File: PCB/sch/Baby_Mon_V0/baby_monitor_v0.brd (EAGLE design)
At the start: 22.8 x 16.2 mm, 2 parts, among them U1 NRF5340-QKAA-AB0-R

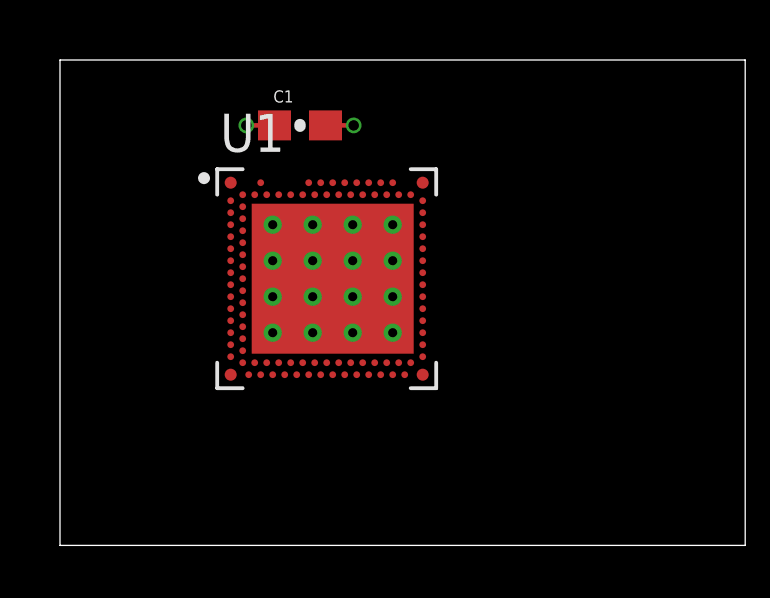
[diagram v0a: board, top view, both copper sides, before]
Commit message: u
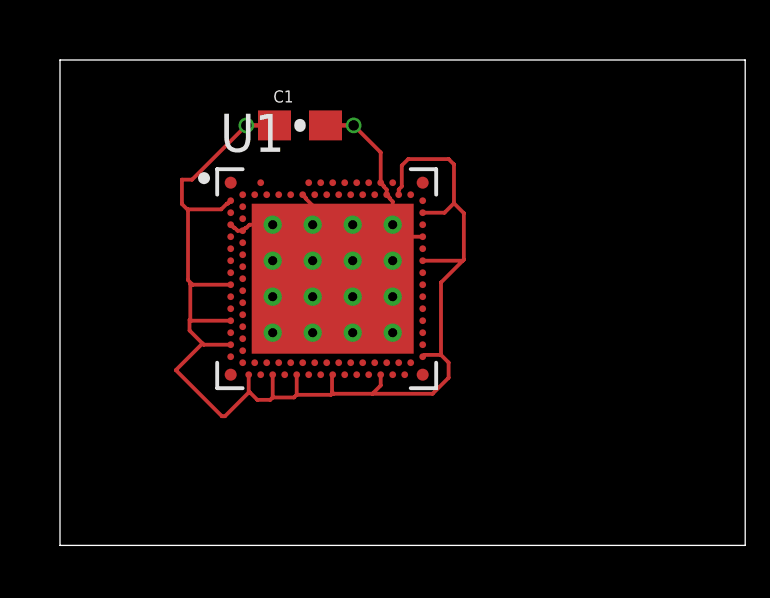
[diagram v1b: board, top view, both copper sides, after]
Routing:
- net 3.3V: track 0.94 -> 43.9 mm
- net GND: track 0.94 -> 8.66 mm

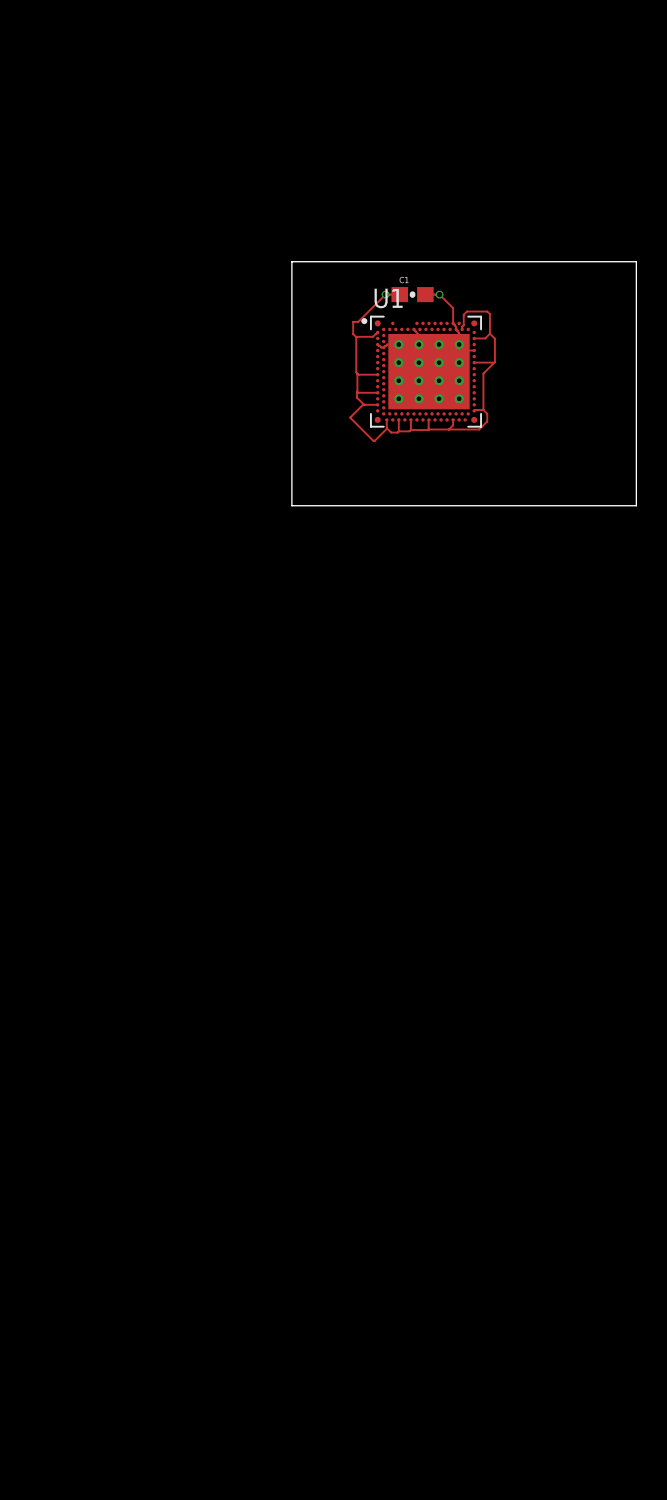
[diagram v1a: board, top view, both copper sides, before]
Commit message: u
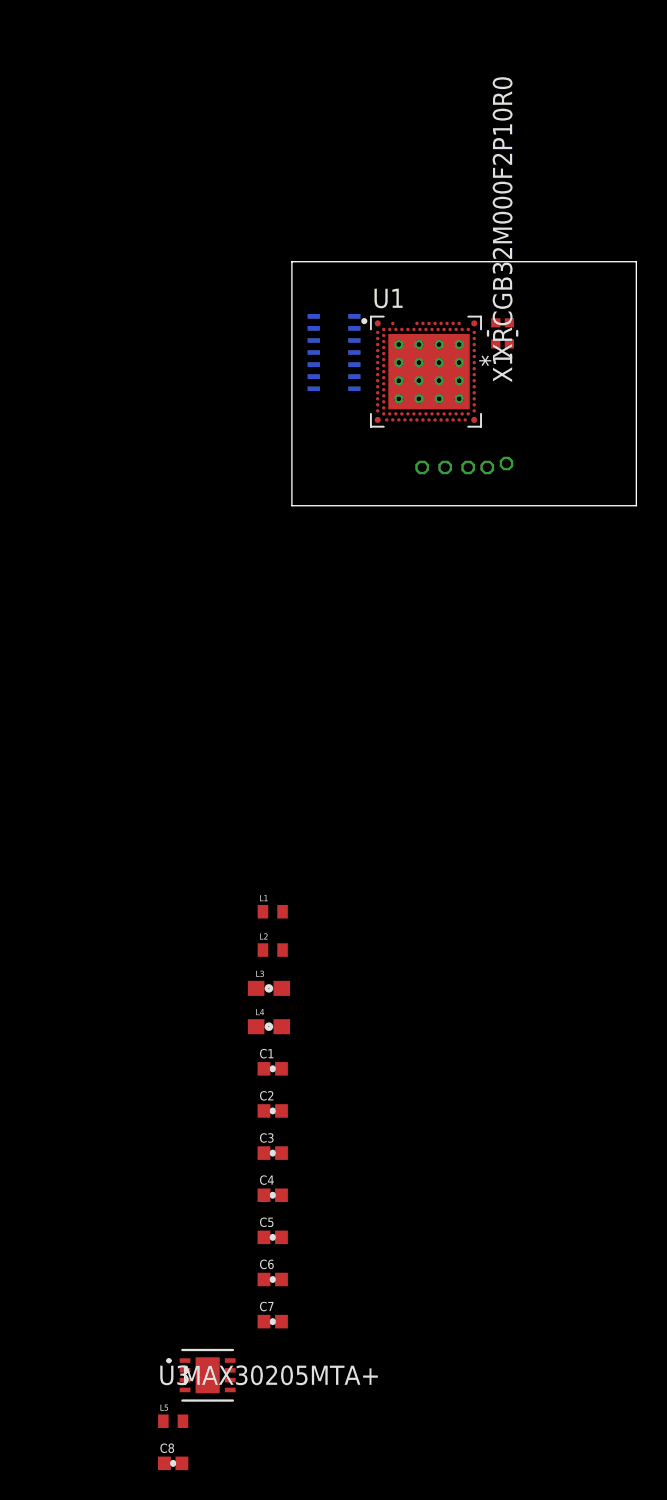
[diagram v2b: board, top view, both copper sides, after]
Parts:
- added C2, C6: 1uF, SparkFun-Capacitors:0402-CAP
- added C3: 1.0uF, SparkFun-Capacitors:0402-CAP
- added C4, C5, C7: 0.1uF, SparkFun-Capacitors:0402-CAP
- added C8: 0.7pF, SparkFun-Capacitors:0402-CAP
- added FRAME1, FRAME2, FRAME3: FRAME-LETTERNO_PACKAGE, SparkFun-Aesthetics:DUMMY
- added J10, J11, J7, J8, J9: (no value), graftel-internal-ic:1X01_TINY
- added L1, L2: 15nH, SparkFun-Passives:C0402
- added L3, L4: 10uH, SparkFun-Passives:0603
- added L5: 2.2nH, SparkFun-Passives:C0402
- added U2: MAX30101EFD+, graftel-internal-ic:21-0880B_MXM
- added U3: MAX30205MTA+, graftel-internal-ic:21-0137_T833+2_MXM
- added X1: XRCGB32M000F2P10R0, graftel-internal-ic:XTAL_SON4_1P6X2P0_MUR
- C1: value (none) -> 1uF; device SparkFun-Capacitors:0603-CAP -> SparkFun-Capacitors:0402-CAP
- moved C1 52.2 mm to (-1.27, -37.3)
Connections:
- removed net DCCD: U1.B10
- removed net DECD: U1.A15
- removed net DECR: U1.A27
- removed net DECRF: U1.G31
- removed net NC: U1.D2, U1.F2, U1.T2
- removed net VDD1: U1.A19
- removed net VDD2: U1.B8
- removed net VDD3: U1.L1
- new net N$1: J11.P$1, U1.AA31
- new net N$10: U1.C31, X1.2
- new net N$11: U1.B30, X1.4
- new net N$12: C8.2, L5.2, U1.L31
- new net N$2: J10.P$1, U1.W31
- new net N$3: J9.P$1, U1.AC31
- new net N$4: L4.2, U1.A21
- new net N$5: L1.2, L4.1
- new net N$6: L2.2, L3.1
- new net N$7: L3.2, U1.B10
- new net N$8: C2.1, L1.1, U1.A27, U1.G31
- new net N$9: C1.1, L2.1, U1.A15
- new net VDD: U2.11, U3.8
- net 3.3V: now also C3.1, C4.1, C5.1, C6.1, C7.1, J8.P$1, U1.A19, U1.B8, U1.L1; no longer C1.1
- net GND: now also C2.2, C3.2, C4.2, C5.2, C6.2, C7.2, C8.1, J7.P$1, X1.1, X1.3
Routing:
- net 3.3V: track 43.9 -> 0.00 mm, vias 1 -> 0
- net GND: track 8.66 -> 0.00 mm, vias 1 -> 0

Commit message: u
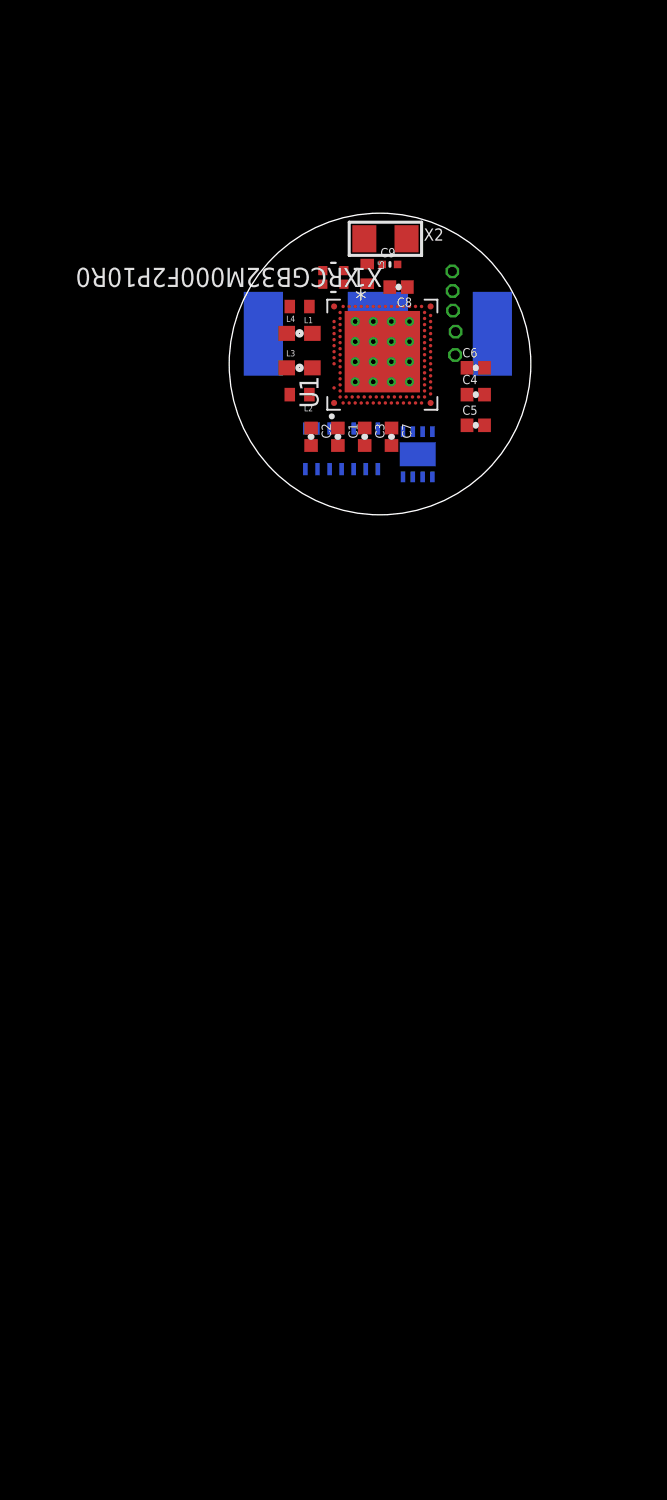
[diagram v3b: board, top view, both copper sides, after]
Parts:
- added C9: (no value), graftel-internal-ic:MICROBUILDER__0402MP
- added J1: BATT-COIN1CR1216, graftel-internal-ic:BC-2017-TR
- added X2: (no value), graftel-internal-ic:ADAFRUIT_WIRELESS_ANT_2450AT18B100
- moved C8 79.4 mm to (7.07, 14.5), turned to 180 degrees
- moved L5 77.2 mm to (4.99, 15.4), turned to 270 degrees
- moved U3 62.6 mm to (8.34, 3.41), flipped to the bottom, turned to 90 degrees
- moved C6 61.9 mm to (12.2, 9.14)
- moved C7 59.2 mm to (6.60, 4.57), turned to 270 degrees
- moved C5 55.5 mm to (12.2, 5.33)
- moved C4 54.8 mm to (12.2, 7.37)
- moved C3 47.9 mm to (4.83, 4.57), turned to 270 degrees
- moved L4 46.0 mm to (0.51, 11.4)
- moved C2 44.8 mm to (1.27, 4.57), turned to 270 degrees
- moved C1 42.1 mm to (3.05, 4.57), turned to 270 degrees
- moved L3 41.2 mm to (0.51, 9.14)
- moved L1 40.2 mm to (0.51, 13.2), turned to 180 degrees
- moved L2 36.9 mm to (0.51, 7.37), turned to 180 degrees
- moved J7 13.2 mm to (10.6, 15.5)
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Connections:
- new net N$13: C9.1, L5.1, X2.FP
- net 3.3V: now also J1.P$2, J1.P$3
- net GND: now also C9.2, J1.P$1
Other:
- board size 22.8 x 16.2 mm -> 20 x 20 mm

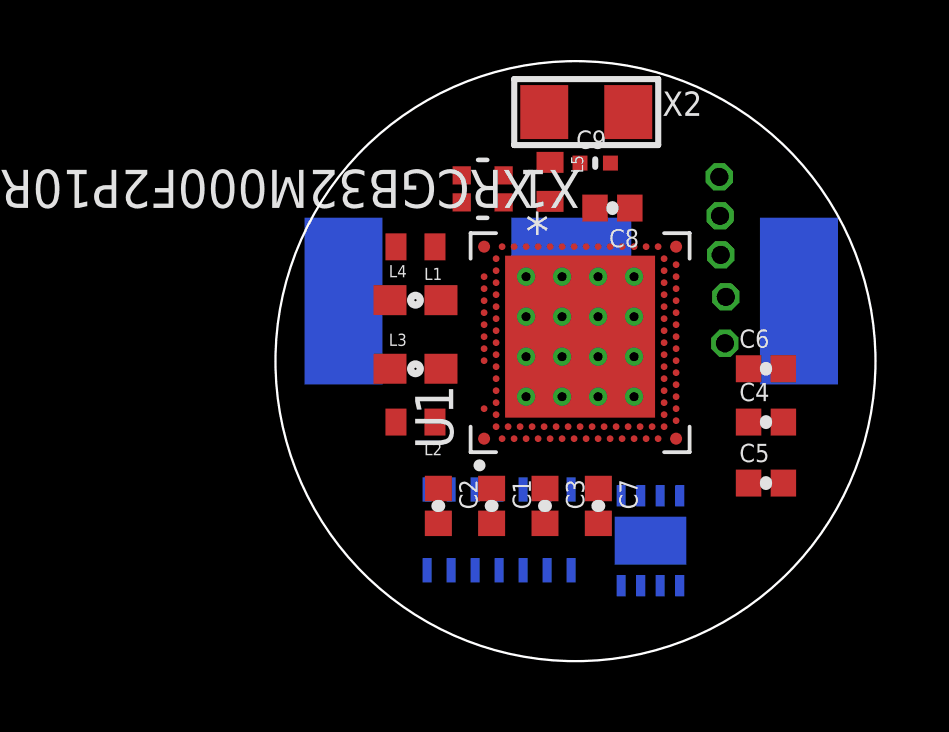
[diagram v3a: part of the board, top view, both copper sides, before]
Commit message: u
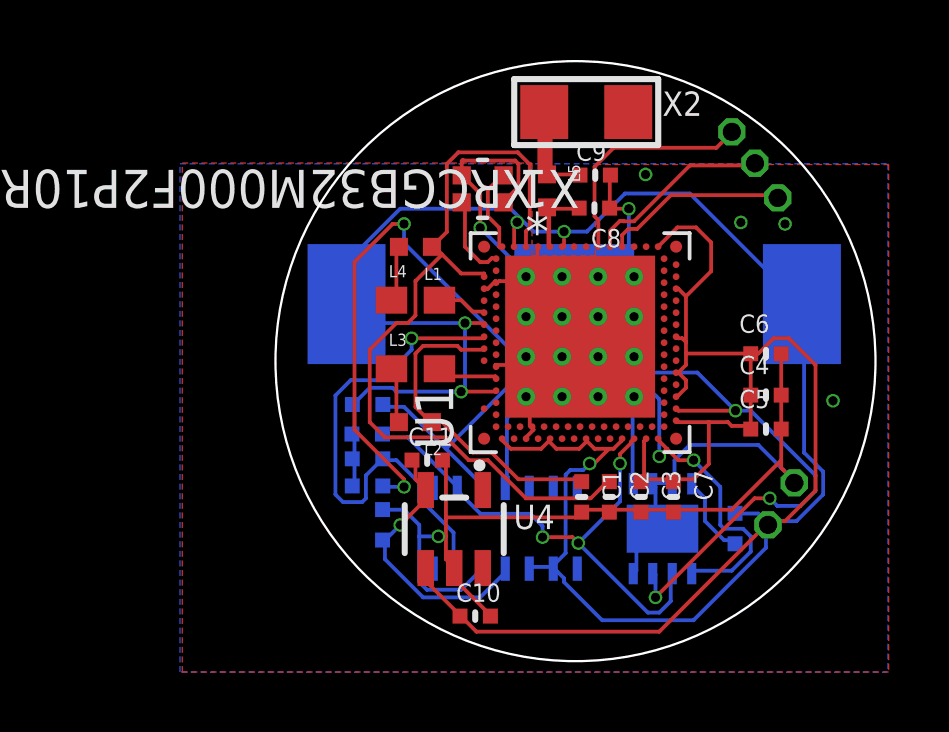
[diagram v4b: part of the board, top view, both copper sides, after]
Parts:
- added C10, C11, C12, C13: 0.1uF, Adafruit Circuit Playground Bluefruit:MICROBUILDER__0402MP
- added R1, R2, R3: 4.7K, Adafruit Circuit Playground Bluefruit:MICROBUILDER__0402MP
- added R4: (no value), Adafruit Circuit Playground Bluefruit:MICROBUILDER__0402MP
- added U4: (no value), Adafruit Circuit Playground Bluefruit:MICROBUILDER_SOT23-5
- C1, C2, C3, C4, C5, C6, C7, C8: device SparkFun-Capacitors:0402-CAP -> Adafruit Circuit Playground Bluefruit:MICROBUILDER__0402MP
- L1, L2, L5: device SparkFun-Passives:C0402 -> Adafruit Circuit Playground Bluefruit:NORDIC_MISC_RESC0402_N
- L3, L4: device SparkFun-Passives:0603 -> Adafruit Circuit Playground Bluefruit:NORDIC_MISC_RESC0603_N
- moved J7 10.5 mm to (13.1, 5.34)
- moved J8 10.4 mm to (12.3, 3.94)
- moved J11 6.08 mm to (11.8, 16.0)
- moved C2 5.71 mm to (6.97, 4.87)
- moved J10 5.50 mm to (11.1, 17.0)
- moved C3 3.21 mm to (8.03, 4.87)
- moved C1 3.01 mm to (6.05, 4.87)
- moved J9 2.69 mm to (12.6, 14.8)
- moved C7 2.52 mm to (9.10, 4.87)
- moved C5 1.80 mm to (12.2, 7.13)
- moved C4 0.90 mm to (12.2, 8.27)
- moved C8 0.60 mm to (6.47, 14.5)
- moved U3 0.57 mm to (8.74, 3.81)
- moved C6 0.50 mm to (12.2, 9.64)
- moved C9 0.40 mm to (6.50, 15.6)
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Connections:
- removed net VDD: U2.11, U3.8
- new net 1.8V: C11.1, C12.2, U2.11, U4.5
- new net 1_8V_EN: U4.3
- new net INT: R3.2, U1.A17, U2.13
- new net N$14: C13.2, U3.8
- new net OS: R4.1, U1.AL5, U3.3
- new net SCL: R2.2, U1.AE1, U2.2, U3.2
- new net SDA: R1.1, U1.AJ1, U2.3, U3.1
- net 3.3V: now also C10.1, C13.1, R1.2, R2.1, R3.1, R4.2, U2.10, U2.9, U4.1
- net GND: now also C10.2, C11.2, C12.1, U2.12, U2.4, U3.4, U3.5, U3.6, U3.7, U3.9, U4.2
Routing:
- net 3.3V: track 0.00 -> 112.1 mm, vias 0 -> 5
- net GND: track 0.00 -> 95.8 mm, vias 0 -> 6
- net OS: track 0.00 -> 39.4 mm, vias 0 -> 5
- net N$8: track 0.00 -> 27.1 mm
- net SDA: track 0.00 -> 23.2 mm, vias 0 -> 2
- net SCL: track 0.00 -> 17.7 mm, vias 0 -> 3
- net INT: track 0.00 -> 17.1 mm, vias 0 -> 1
- net N$9: track 0.00 -> 10.8 mm
- net 1.8V: track 0.00 -> 9.28 mm, vias 0 -> 1
- net N$2: track 0.00 -> 7.80 mm
- net N$1: track 0.00 -> 6.35 mm
- net N$3: track 0.00 -> 6.16 mm
- net N$13: track 0.00 -> 3.21 mm
- net N$10: track 0.00 -> 2.91 mm
- net N$11: track 0.00 -> 2.84 mm
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- added copper zone on layer 1, net GND
- added copper zone on layer 16, net GND
